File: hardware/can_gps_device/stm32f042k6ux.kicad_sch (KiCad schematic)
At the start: 20 parts, among them J2 TC2030, U1 STM32F042K6Ux, Y1 ECS-160-10-36Q-AES-TR

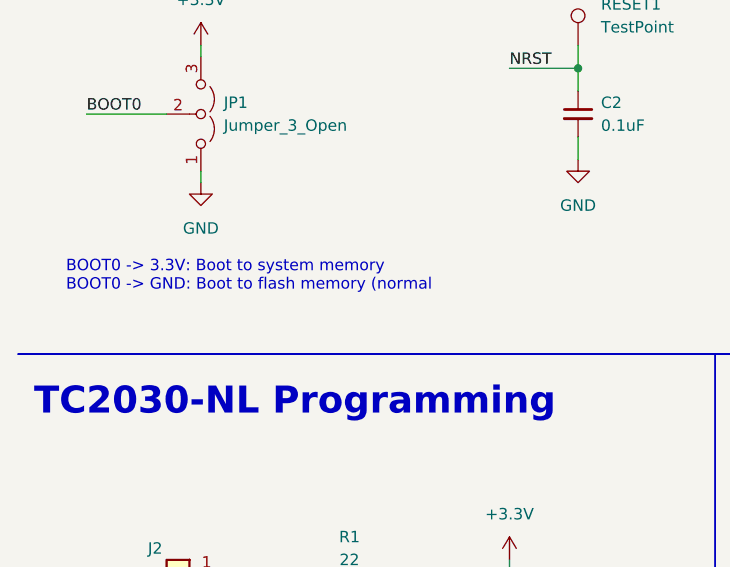
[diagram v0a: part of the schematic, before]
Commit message: Updated MX config and schematic PDF
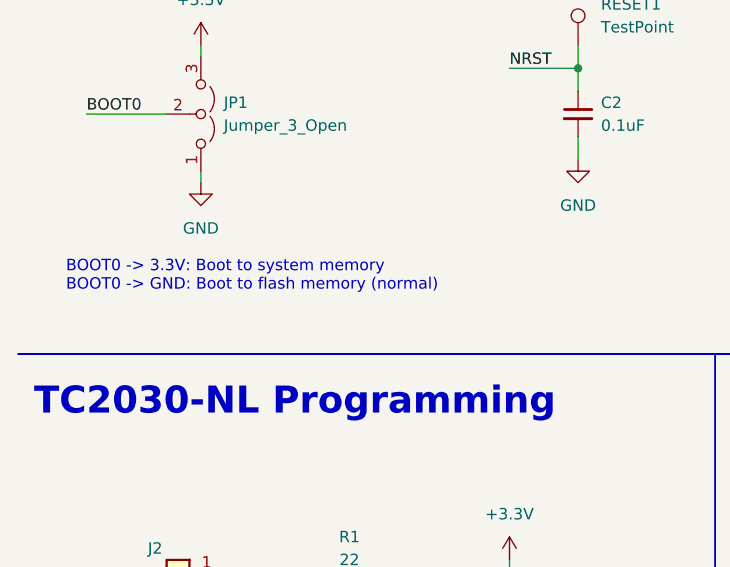
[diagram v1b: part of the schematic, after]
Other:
- note added: "BOOT0 -> 3.3V: Boot to system memory BOOT0 -> GND: Boot to flash memory (normal)"
- note removed: "BOOT0 -> 3.3V: Boot to system memory BOOT0 -> GND: Boot to flash memory (normal"
